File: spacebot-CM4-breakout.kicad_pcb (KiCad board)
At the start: 2 copper layers, 2 parts, among them J1 Conn_02x12_Counter_Clockwise, U1 Compute_Module_4_Connectors

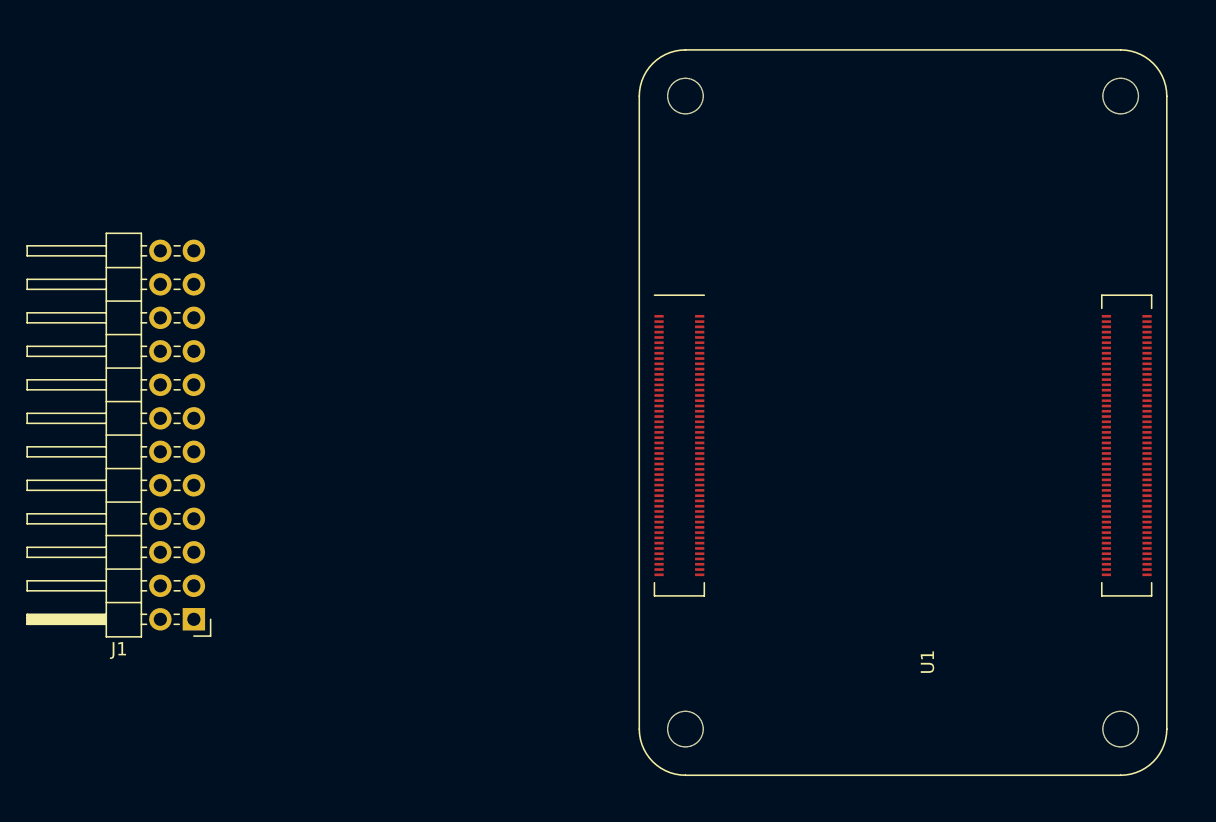
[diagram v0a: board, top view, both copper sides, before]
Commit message: updates
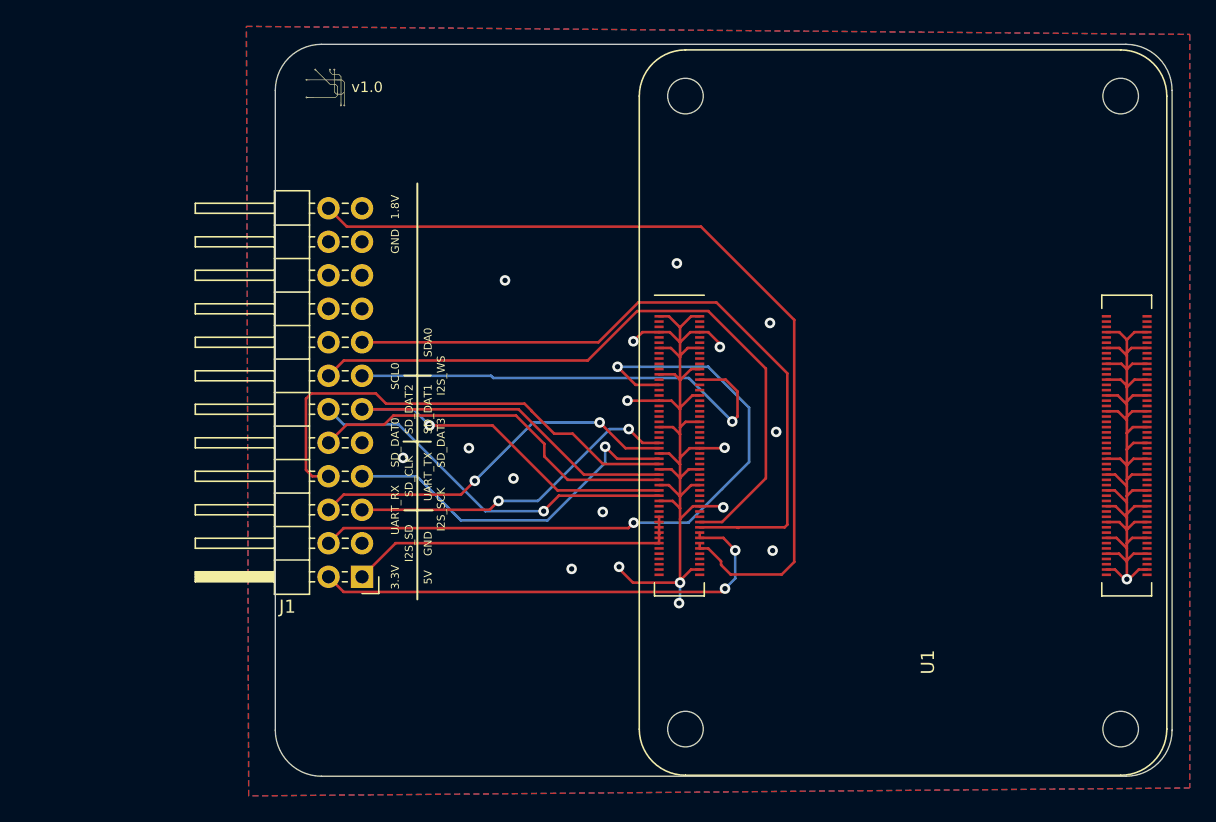
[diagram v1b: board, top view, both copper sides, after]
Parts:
- added G***: LOGO, trylaarsdam:wcl_logo, F.Cu at (106.6, 74.3)
- moved J1 13.2 mm to (110.1, 111.4)
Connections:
- U1 pad 61: SD_DAT1 -> SD_DAT3
- U1 pad 63: SD_DAT2 -> SD_DAT0
- U1 pad 67: unconnected-(U1-Pad67) -> SD_DAT1
- U1 pad 69: unconnected-(U1-Pad69) -> SD_DAT2
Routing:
- net GND: track 0.00 -> 147.2 mm, vias 0 -> 19
- net 1.8V: track 0.00 -> 66.1 mm
- net SDA_0: track 0.00 -> 54.0 mm
- net I2S_SD: track 0.00 -> 53.5 mm, vias 0 -> 2
- net SCL_0: track 0.00 -> 51.7 mm
- net 3.3V: track 0.00 -> 37.4 mm, vias 0 -> 2
- net SD_CLK: track 0.00 -> 36.5 mm
- net I2S_WS: track 0.00 -> 35.2 mm, vias 0 -> 1
- net SD_DAT2: track 0.00 -> 28.8 mm, vias 0 -> 1
- net UART_RX: track 0.00 -> 28.6 mm, vias 0 -> 2
- net SD_DAT0: track 0.00 -> 28.5 mm
- net UART_TX: track 0.00 -> 27.3 mm, vias 0 -> 1
- net 5V: track 0.00 -> 25.7 mm
- net I2S_SCK: track 0.00 -> 25.5 mm, vias 0 -> 2
- net SD_DAT1: track 0.00 -> 25.1 mm, vias 0 -> 1
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- added copper zone on B.Cu, net GND
- added copper zone on F.Cu, net GND
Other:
- board outline added: 68 x 55.5 mm
- board text added: "1.8V"
- board text added: "3.3V"
- board text added: "5V"
- board text added: "GND"
- board text added: "I2S_SCK"
- board text added: "I2S_SD"
- board text added: "I2S_WS"
- board text added: "SCL0"
- board text added: "SDA0"
- board text added: "SD_CLK"
- board text added: "SD_DAT0"
- board text added: "SD_DAT1"
- board text added: "SD_DAT2"
- board text added: "SD_DAT3"
- board text added: "UART_RX"
- board text added: "UART_TX"
- board text added: "v1.0"
